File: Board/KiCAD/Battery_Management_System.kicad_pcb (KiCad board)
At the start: 4 copper layers, 47.7 x 62.6 mm, 117 parts, among them J1 Conn_01x06_Socket, J10 Conn_01x02, J11 Conn_01x02, J12 Conn_01x02, J13 Conn_01x02, J2 Conn_ARM_SWD_TagConnect_TC2030, J4 Conn_01x03, J5 Conn_01x03, J7 Conn_01x05, J8 Conn_01x02, J9 Conn_01x02, Q1 AON7408, Q10 AON7407, Q2 AON7408, Q23 2N7002, Q24 2N7002, Q25 2N7002, Q26 2N7002, Q3 AON7408, Q4 AON7408, Q5 BSS83P, Q6 BSS83P, Q7 BSS83P, Q8 BSS83P, SW2 SW_Push, U1 BQ25730RSNR, U10 INA219BxD, U2 INA219BxD, U3 LTC2943CDD#PBF, U4 INA219BxD, U5 LMR50410, U9 STM32F103C8T6, Y1 Crystal_GND24_Small, Y4 CM8V-T1A-32.768KHZ-12.5PF-20P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

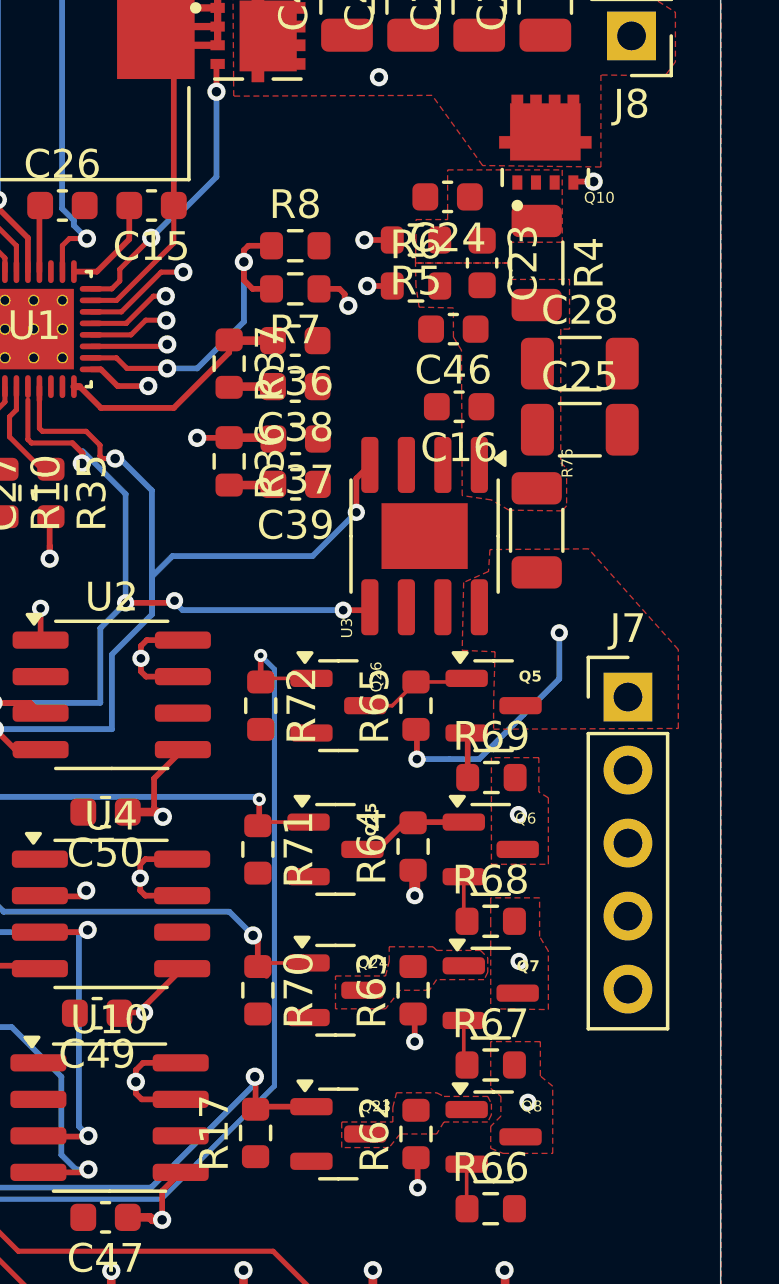
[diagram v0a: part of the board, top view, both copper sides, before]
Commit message: more updates
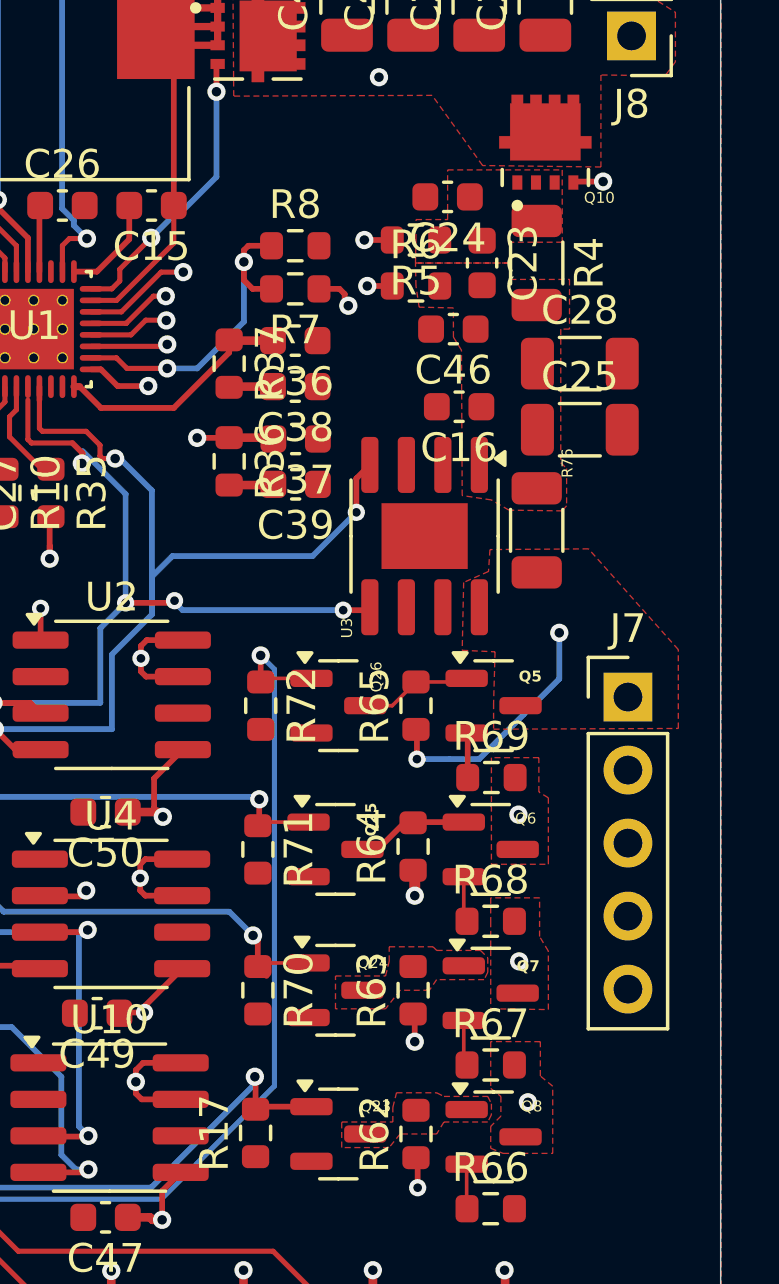
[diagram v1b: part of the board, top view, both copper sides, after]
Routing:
- net GND: track 24.3 -> 4.28 mm
- net Net-(U9-PC14-OSC32_IN): track 19.8 -> 8.66 mm
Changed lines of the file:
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@@
 	)
 	(segment
-		(start 216.5 72)
-		(end 216.5 74.74)
-		(width 0.127)
-		(layer "In1.Cu")
-		(net 1)
-	)
-	(segment
-		(start 224 83.5)
-		(end 224 82.24)
-		(width 0.127)
-		(layer "In1.Cu")
-		(net 1)
-	)
-	(segment
-		(start 216.5 74.74)
-		(end 218.5 76.74)
-		(width 0.127)
-		(layer "In1.Cu")
-		(net 1)
-	)
-	(segment
-		(start 217.14 78.1)
-		(end 218.5 76.74)
-		(width 0.127)
-		(layer "In1.Cu")
-		(net 1)
-	)
-	(segment
-		(start 214.35 77)
-		(end 215.45 78.1)
-		(width 0.127)
-		(layer "In1.Cu")
-		(net 1)
-	)
-	(segment
-		(start 214.0712 77.0128)
-		(end 214.084 77)
-		(width 0.127)
-		(layer "In1.Cu")
-		(net 1)
-	)
-	(segment
-		(start 214.084 77)
-		(end 214.35 77)
-		(width 0.127)
-		(layer "In1.Cu")
-		(net 1)
-	)
-	(segment
-		(start 215.45 78.1)
-		(end 217.14 78.1)
-		(width 0.127)
-		(layer "In1.Cu")
-		(net 1)
-	)
-	(segment
-		(start 224 82.24)
-		(end 218.5 76.74)
-		(width 0.127)
-		(layer "In1.Cu")
-		(net 1)
-	)
-	(segment
 		(start 214.35 54.75)
 		(end 214.8 55.2)
@@
 	)
 	(segment
-		(start 210 84.625)
-		(end 206.625 88)
-		(width 0.127)
-		(layer "In1.Cu")
-		(net 13)
-	)
-	(segment
-		(start 209.7278 78.3844)
-		(end 210 78.6566)
-		(width 0.127)
-		(layer "In1.Cu")
-		(net 13)
-	)
-	(segment
-		(start 210 78.6566)
-		(end 210 84.625)
-		(width 0.127)
-		(layer "In1.Cu")
-		(net 13)
-	)
-	(segment
 		(start 211.895 82.85)
 		(end 213.2028 82.85)
@@
 	)
 	(segment
-		(start 246.38 59.8678)
-		(end 245.7072 59.8678)
-		(width 0.2)
-		(layer "F.Cu")
-		(net 34)
-	)
-	(segment
 		(start 231.065657 63.853243)
 		(end 230.1189 64.8)
@@
 	)
 	(segment
-		(start 230.1189 64.8)
-		(end 228.9 64.8)
-		(width 0.1778)
+		(start 246.7102 59.8678)
+		(end 245.7072 59.8678)
+		(width 0.2)
 		(layer "F.Cu")
 		(net 34)
@@
 	)
 	(segment
+		(start 230.1189 64.8)
+		(end 228.9 64.8)
+		(width 0.1778)
+		(layer "F.Cu")
+		(net 34)
+	)
+	(segment
 		(start 231.4956 63.853243)
 		(end 231.065657 63.853243)
@@
 	)
 	(via
-		(at 246.38 59.8678)
+		(at 246.7102 59.8678)
 		(size 0.635)
 		(drill 0.3302)
@@
 	)
 	(segment
-		(start 233.2482 62.749092)
-		(end 233.2482 58.4791)
+		(start 233.2482 58.501586)
+		(end 233.2482 62.749092)
 		(width 0.1778)
 		(layer "In2.Cu")
@@
 	)
 	(segment
-		(start 232.144049 63.853243)
-		(end 233.2482 62.749092)
+		(start 234.675986 57.0738)
+		(end 233.2482 58.501586)
 		(width 0.1778)
 		(layer "In2.Cu")
@@
 	)
 	(segment
-		(start 233.2482 58.4791)
-		(end 234.6535 57.0738)
+		(start 246.38 59.5376)
+		(end 246.38 57.7596)
 		(width 0.1778)
 		(layer "In2.Cu")
@@
 	(segment
 		(start 246.38 57.7596)
-		(end 246.38 59.8678)
+		(end 245.6942 57.0738)
 		(width 0.1778)
 		(layer "In2.Cu")
@@
 	)
 	(segment
-		(start 245.6942 57.0738)
-		(end 246.38 57.7596)
+		(start 233.2482 62.749092)
+		(end 232.144049 63.853243)
 		(width 0.1778)
 		(layer "In2.Cu")
@@
 	)
 	(segment
-		(start 234.6535 57.0738)
-		(end 245.6942 57.0738)
+		(start 232.144049 63.853243)
+		(end 231.4956 63.853243)
 		(width 0.1778)
 		(layer "In2.Cu")
@@
 	)
 	(segment
-		(start 231.4956 63.853243)
-		(end 232.144049 63.853243)
+		(start 245.6942 57.0738)
+		(end 234.675986 57.0738)
+		(width 0.1778)
+		(layer "In2.Cu")
+		(net 34)
+	)
+	(segment
+		(start 246.7102 59.8678)
+		(end 246.38 59.5376)
 		(width 0.1778)
 		(layer "In2.Cu")
@@
 	(via
 		(at 234.7468 81.3562)
-		(size 0.4572)
-		(drill 0.2032)
+		(size 0.635)
+		(drill 0.3302)
 		(layers "F.Cu" "B.Cu")
 		(free yes)
@@
 	(via
 		(at 234.7976 76.3524)
-		(size 0.4572)
-		(drill 0.2032)
+		(size 0.635)
+		(drill 0.3302)
 		(layers "F.Cu" "B.Cu")
 		(free yes)
@@
 	(via
 		(at 244.094 91.8972)
-		(size 0.6)
-		(drill 0.3)
+		(size 0.635)
+		(drill 0.3302)
 		(layers "F.Cu" "B.Cu")
 		(free yes)
@@
 	(via
 		(at 240.157 89.789)
-		(size 0.6)
-		(drill 0.3)
+		(size 0.635)
+		(drill 0.3302)
 		(layers "F.Cu" "B.Cu")
 		(net 44)
@@
 	(via
 		(at 243.7892 86.995)
-		(size 0.6)
-		(drill 0.3)
+		(size 0.635)
+		(drill 0.3302)
 		(layers "F.Cu" "B.Cu")
 		(free yes)
@@
 	(via
 		(at 243.7638 81.8896)
-		(size 0.6)
-		(drill 0.3)
+		(size 0.635)
+		(drill 0.3302)
 		(layers "F.Cu" "B.Cu")
 		(free yes)
@@
 	(via
 		(at 240.157 84.709)
-		(size 0.6)
-		(drill 0.3)
+		(size 0.635)
+		(drill 0.3302)
 		(layers "F.Cu" "B.Cu")
 		(net 45)
@@
 	(via
 		(at 245.1862 75.565)
-		(size 0.6)
-		(drill 0.3)
+		(size 0.635)
+		(drill 0.3302)
 		(layers "F.Cu" "B.Cu")
 		(free yes)
